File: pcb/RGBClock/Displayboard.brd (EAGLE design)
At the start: 70 x 58.5 mm, 66 parts, among them IC1 MCP23017SO, U1 LP3878MR-ADJ, U2 P82B96DR, U3 P82B96DR, U4 PCA9685PW, U5 TPS71533DCKR, U6 ZXLD1362ET5TA, U7 74HCT1G14GW, U8 74HCT1G86GW, X1 43045-0400, X2 43045-0400, X3 43045-0400, X4 1503_09

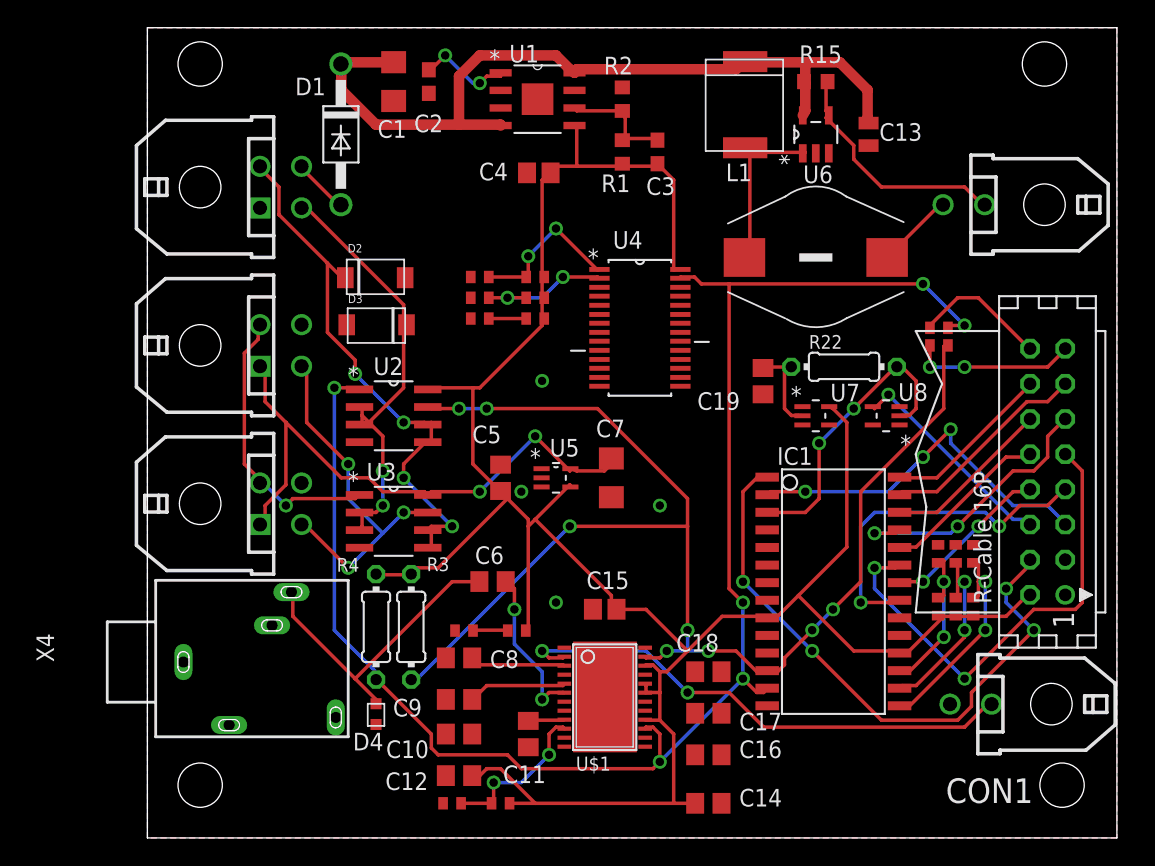
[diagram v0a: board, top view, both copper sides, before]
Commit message: Just before freerouter
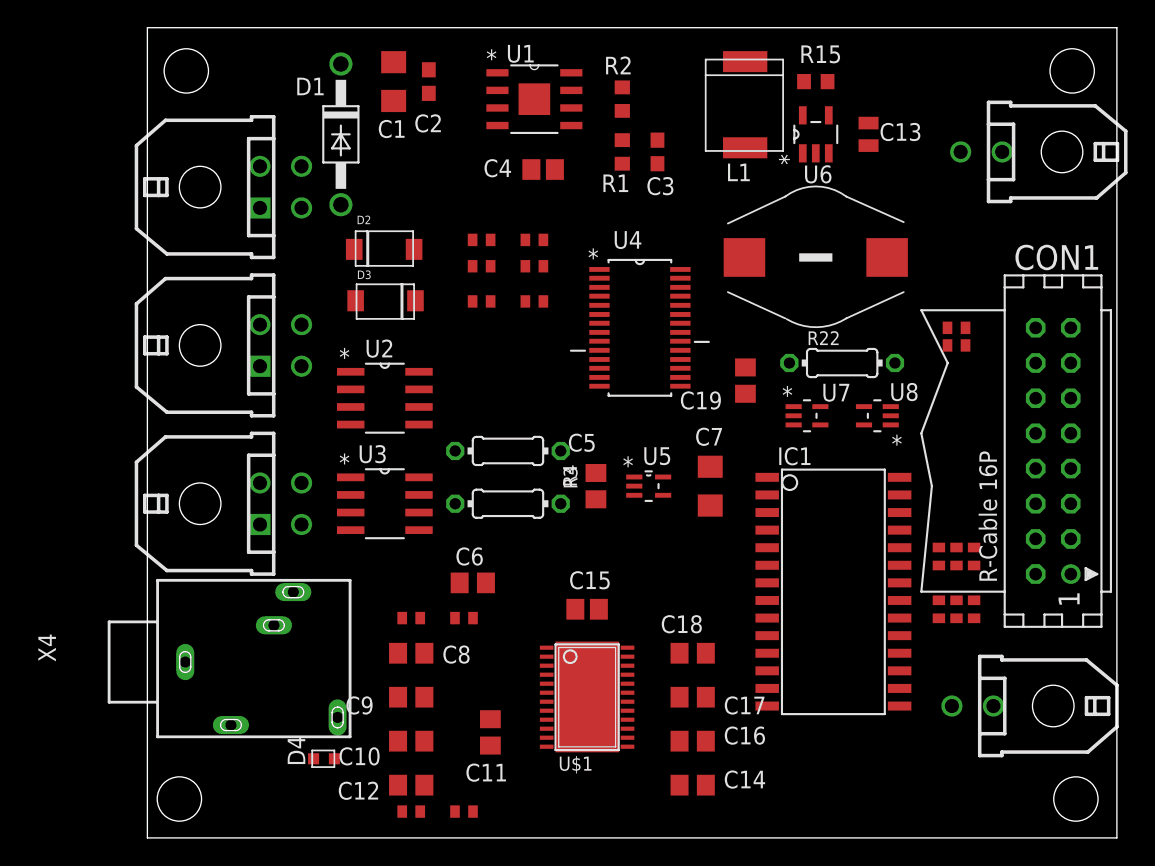
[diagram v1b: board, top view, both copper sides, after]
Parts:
- moved R3 14.5 mm to (26.0, 27.9), turned to 0 degrees
- moved R4 13.0 mm to (26.0, 24.1), turned to 0 degrees
- moved C7 7.17 mm to (40.6, 25.4)
- moved C5 6.91 mm to (32.4, 25.4)
- moved U5 6.72 mm to (36.2, 25.4)
- moved D4 4.96 mm to (12.7, 5.71), turned to 180 degrees
- moved X6 4.02 mm to (66.0, 49.5)
- moved R13 3.92 mm to (22.9, 15.9)
- moved R14 3.92 mm to (19.1, 15.9)
- moved C12 3.52 mm to (19.1, 3.81)
- moved C10 3.49 mm to (19.1, 6.99)
- moved C8 3.47 mm to (19.1, 13.3)
- moved C9 3.45 mm to (19.1, 10.2)
- moved R12 3.01 mm to (19.1, 1.91)
- moved C11 2.74 mm to (24.8, 7.62)
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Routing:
- net +5V: track 175.3 -> 0.00 mm
- net SDA: track 115.1 -> 0.00 mm, vias 6 -> 0
- net SCL: track 96.2 -> 0.00 mm, vias 8 -> 0
- net VCC: track 60.0 -> 0.00 mm
- net RS: track 44.0 -> 0.00 mm, vias 4 -> 0
- net +3V3: track 42.3 -> 0.00 mm, vias 2 -> 0
- net N$22: track 40.1 -> 0.00 mm, vias 4 -> 0
- net N$12: track 37.2 -> 0.00 mm, vias 2 -> 0
- net D2: track 34.6 -> 0.00 mm, vias 2 -> 0
- net N$2: track 32.5 -> 0.00 mm, vias 2 -> 0
- net RW: track 26.9 -> 0.00 mm, vias 3 -> 0
- net N$9: track 26.7 -> 0.00 mm, vias 3 -> 0
- net D0: track 25.0 -> 0.00 mm, vias 2 -> 0
- net N$49: track 22.4 -> 0.00 mm
- net N$3: track 21.3 -> 0.00 mm, vias 2 -> 0
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- removed copper zone on layer 1, net GND
- removed copper zone on layer 16, net GND
